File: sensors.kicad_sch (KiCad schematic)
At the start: 9 parts, among them IC4 BME690, U2 BME280, U3 BMP581

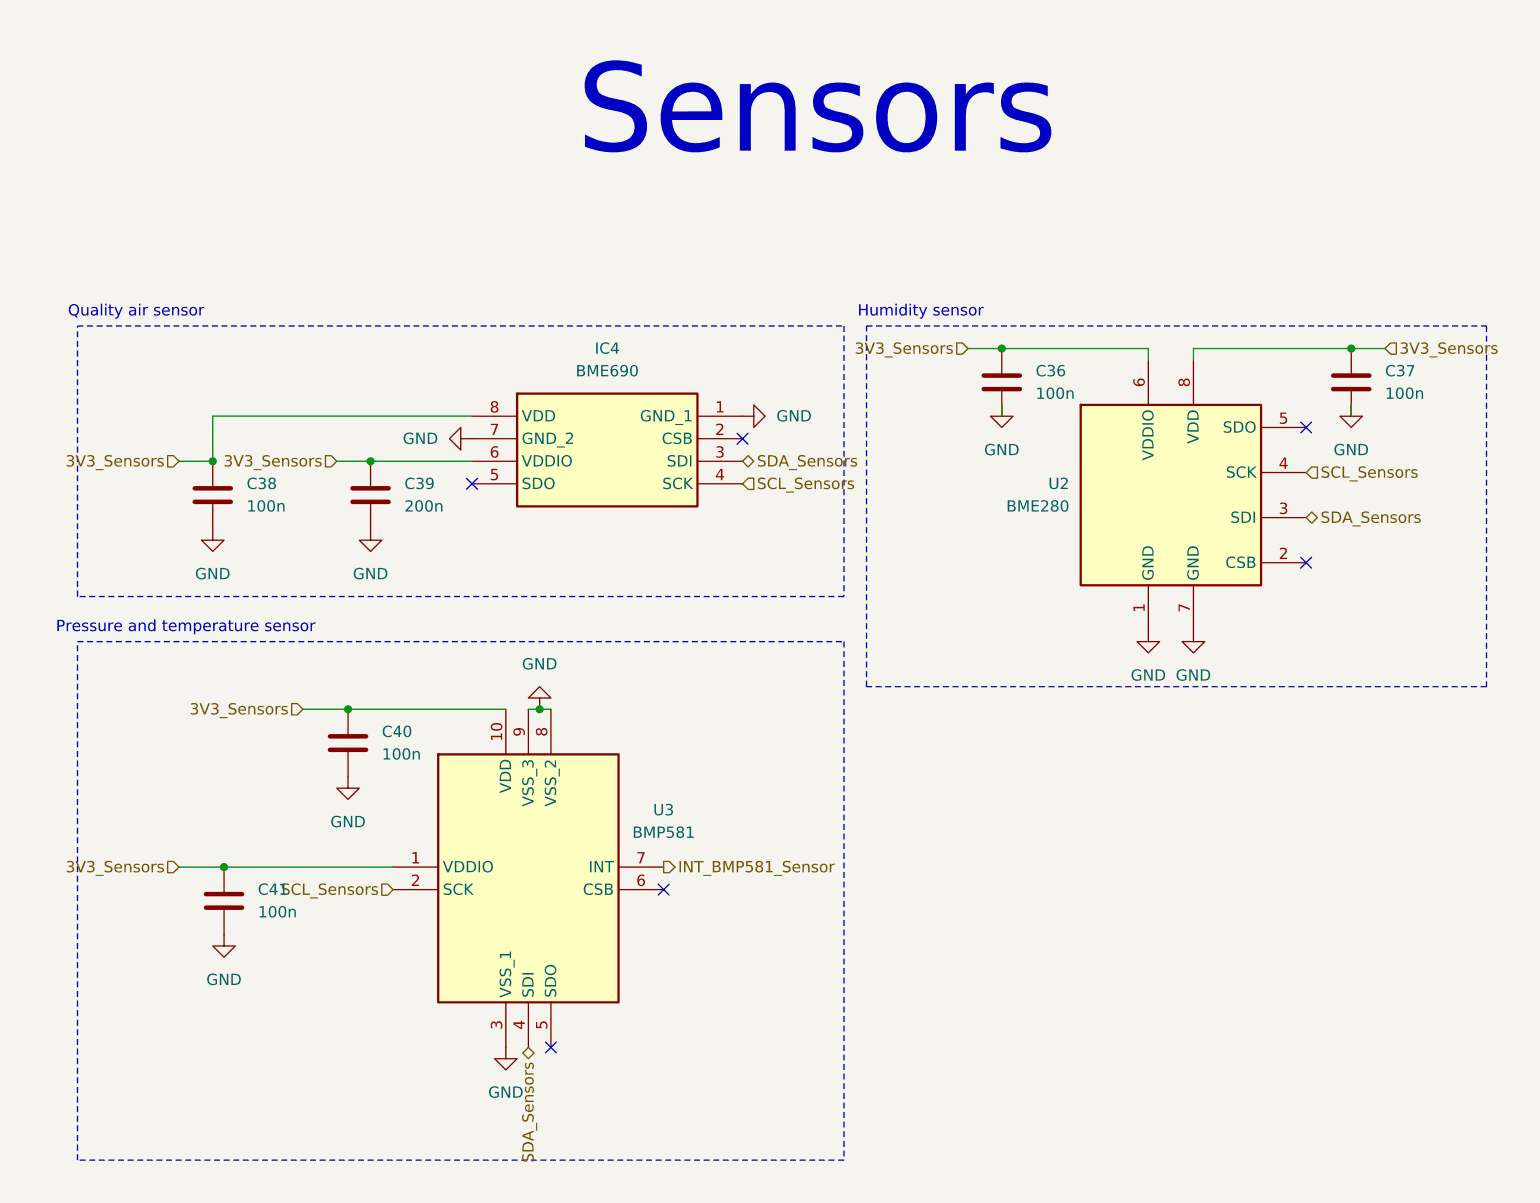
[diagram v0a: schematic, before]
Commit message: Place all components on the PCB correctly
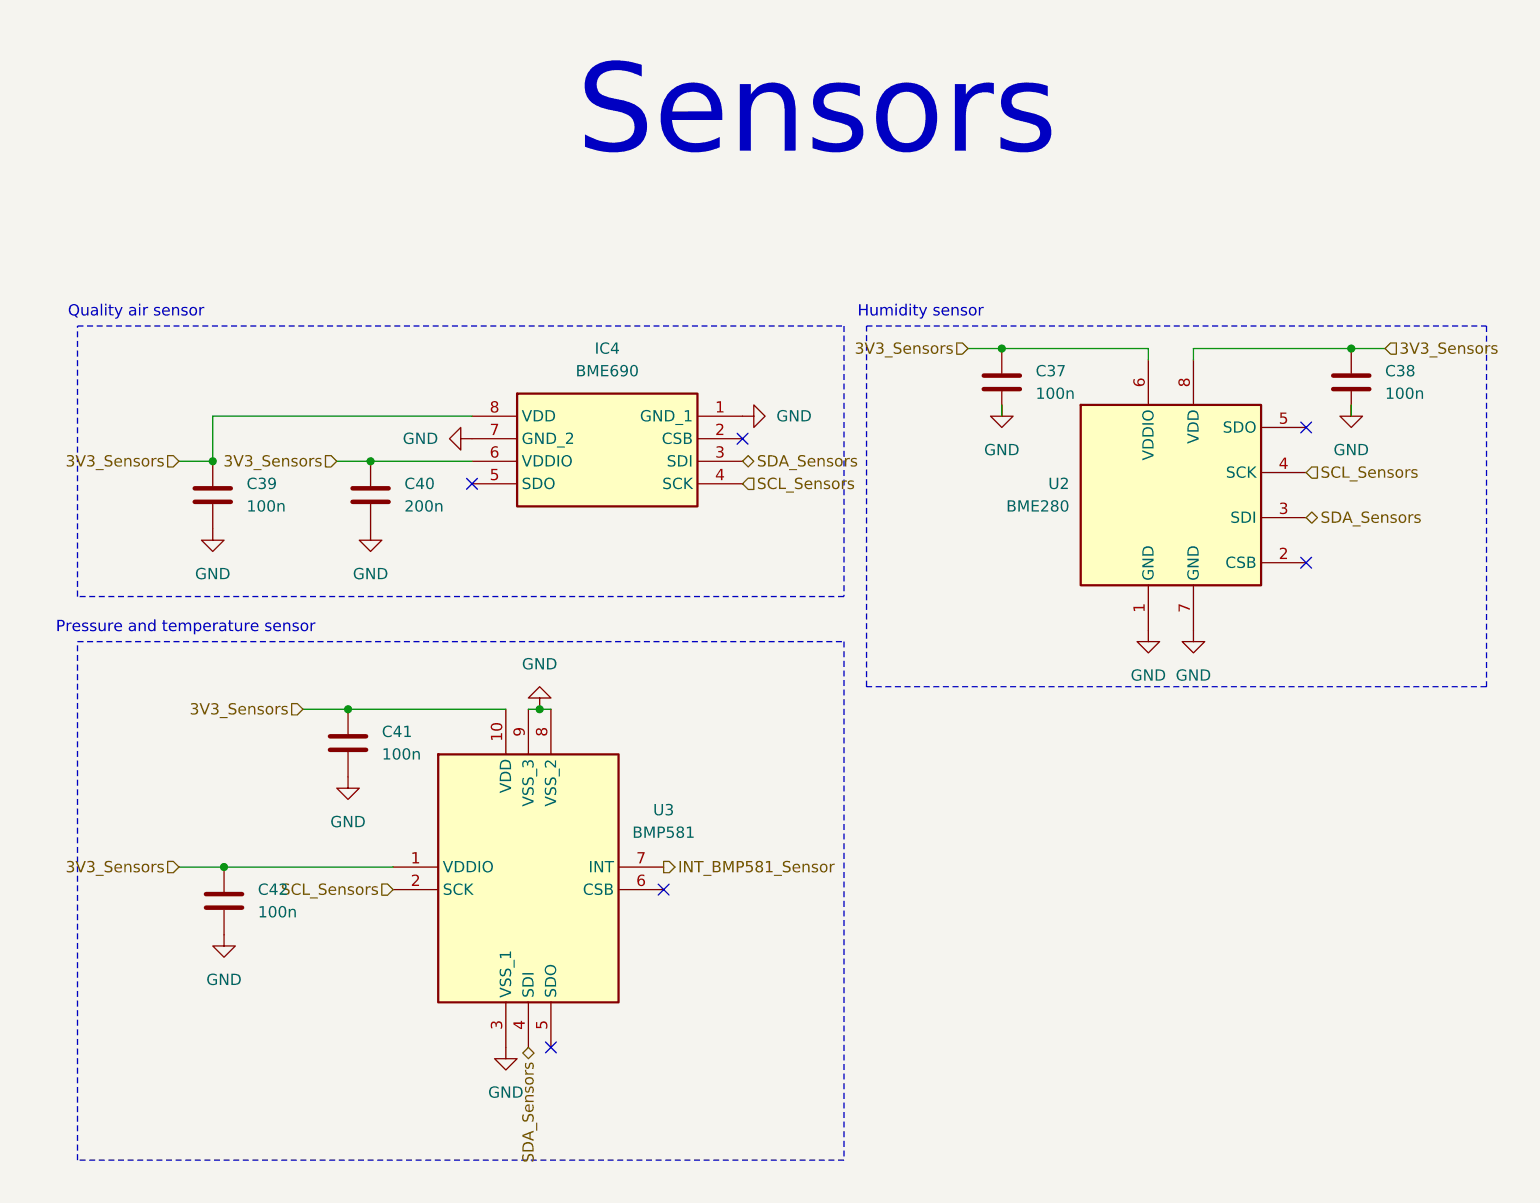
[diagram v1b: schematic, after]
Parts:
- renumbered C36 to C37, C37 to C38, C38 to C39, C39 to C40, C40 to C41, C41 to C42
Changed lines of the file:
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@@
 		(dnp no)
 		(fields_autoplaced yes)
-		(property "Reference" "#PWR058"
+		(property "Reference" "#PWR059"
 			(at 170.18 66.04 0)
 			(effects
@@
 			(project "weather-station-poc"
 				(path "/38eb53bb-294e-46e4-ad59-fd355ca373b9/29574217-d56b-4a63-a2c4-128dfec2758e"
-					(reference "#PWR058")
+					(reference "#PWR059")
 					(unit 1)
 				)
@@
 		(dnp no)
 		(fields_autoplaced yes)
-		(property "Reference" "#PWR060"
+		(property "Reference" "#PWR061"
 			(at 147.32 60.96 0)
 			(effects
@@
 			(project "weather-station-poc"
 				(path "/38eb53bb-294e-46e4-ad59-fd355ca373b9/29574217-d56b-4a63-a2c4-128dfec2758e"
-					(reference "#PWR060")
+					(reference "#PWR061")
 					(unit 1)
 				)
@@
 		(dnp no)
 		(fields_autoplaced yes)
-		(property "Reference" "C37"
+		(property "Reference" "C38"
 			(at 213.36 55.8799 0)
 			(effects
@@
 			(project "weather-station-poc"
 				(path "/38eb53bb-294e-46e4-ad59-fd355ca373b9/29574217-d56b-4a63-a2c4-128dfec2758e"
-					(reference "C37")
+					(reference "C38")
 					(unit 1)
 				)
@@
 		(dnp no)
 		(fields_autoplaced yes)
-		(property "Reference" "C38"
+		(property "Reference" "C39"
 			(at 85.09 68.5799 0)
 			(effects
@@
 			(project ""
 				(path "/38eb53bb-294e-46e4-ad59-fd355ca373b9/29574217-d56b-4a63-a2c4-128dfec2758e"
-					(reference "C38")
+					(reference "C39")
 					(unit 1)
 				)
@@
 		(dnp no)
 		(fields_autoplaced yes)
-		(property "Reference" "#PWR062"
+		(property "Reference" "#PWR063"
 			(at 81.28 80.01 0)
 			(effects
@@
 			(project ""
 				(path "/38eb53bb-294e-46e4-ad59-fd355ca373b9/29574217-d56b-4a63-a2c4-128dfec2758e"
-					(reference "#PWR062")
+					(reference "#PWR063")
 					(unit 1)
 				)
@@
 		(dnp no)
 		(fields_autoplaced yes)
-		(property "Reference" "#PWR065"
+		(property "Reference" "#PWR066"
 			(at 191.77 91.44 0)
 			(effects
@@
 			(project "weather-station-poc"
 				(path "/38eb53bb-294e-46e4-ad59-fd355ca373b9/29574217-d56b-4a63-a2c4-128dfec2758e"
-					(reference "#PWR065")
+					(reference "#PWR066")
 					(unit 1)
 				)
@@
 		(dnp no)
 		(fields_autoplaced yes)
-		(property "Reference" "#PWR066"
+		(property "Reference" "#PWR067"
 			(at 118.11 87.63 0)
 			(effects
@@
 			(project "weather-station-poc"
 				(path "/38eb53bb-294e-46e4-ad59-fd355ca373b9/29574217-d56b-4a63-a2c4-128dfec2758e"
-					(reference "#PWR066")
+					(reference "#PWR067")
 					(unit 1)
 				)
@@
 		(dnp no)
 		(fields_autoplaced yes)
-		(property "Reference" "C39"
+		(property "Reference" "C40"
 			(at 102.87 68.5799 0)
 			(effects
@@
 			(project "weather-station-poc"
 				(path "/38eb53bb-294e-46e4-ad59-fd355ca373b9/29574217-d56b-4a63-a2c4-128dfec2758e"
-					(reference "C39")
+					(reference "C40")
 					(unit 1)
 				)
@@
 		(dnp no)
 		(fields_autoplaced yes)
-		(property "Reference" "#PWR063"
+		(property "Reference" "#PWR064"
 			(at 99.06 80.01 0)
 			(effects
@@
 			(project "weather-station-poc"
 				(path "/38eb53bb-294e-46e4-ad59-fd355ca373b9/29574217-d56b-4a63-a2c4-128dfec2758e"
-					(reference "#PWR063")
+					(reference "#PWR064")
 					(unit 1)
 				)
@@
 		(dnp no)
 		(fields_autoplaced yes)
-		(property "Reference" "#PWR059"
+		(property "Reference" "#PWR060"
 			(at 209.55 66.04 0)
 			(effects
@@
 			(project "weather-station-poc"
 				(path "/38eb53bb-294e-46e4-ad59-fd355ca373b9/29574217-d56b-4a63-a2c4-128dfec2758e"
-					(reference "#PWR059")
+					(reference "#PWR060")
 					(unit 1)
 				)
@@
 		(dnp no)
 		(fields_autoplaced yes)
-		(property "Reference" "#PWR068"
+		(property "Reference" "#PWR069"
 			(at 82.55 125.73 0)
 			(effects
@@
 			(project "weather-station-poc"
 				(path "/38eb53bb-294e-46e4-ad59-fd355ca373b9/29574217-d56b-4a63-a2c4-128dfec2758e"
-					(reference "#PWR068")
+					(reference "#PWR069")
 					(unit 1)
 				)
@@
 		(dnp no)
 		(fields_autoplaced yes)
-		(property "Reference" "#PWR067"
+		(property "Reference" "#PWR068"
 			(at 96.52 107.95 0)
 			(effects
@@
 			(project "weather-station-poc"
 				(path "/38eb53bb-294e-46e4-ad59-fd355ca373b9/29574217-d56b-4a63-a2c4-128dfec2758e"
-					(reference "#PWR067")
+					(reference "#PWR068")
 					(unit 1)
 				)
@@
 		(dnp no)
 		(fields_autoplaced yes)
-		(property "Reference" "#PWR069"
+		(property "Reference" "#PWR070"
 			(at 114.3 138.43 0)
 			(effects
@@
 			(project "weather-station-poc"
 				(path "/38eb53bb-294e-46e4-ad59-fd355ca373b9/29574217-d56b-4a63-a2c4-128dfec2758e"
-					(reference "#PWR069")
+					(reference "#PWR070")
 					(unit 1)
 				)
@@
 		(dnp no)
 		(fields_autoplaced yes)
-		(property "Reference" "#PWR061"
+		(property "Reference" "#PWR062"
 			(at 104.14 63.5 0)
 			(effects
@@
 			(project "weather-station-poc"
 				(path "/38eb53bb-294e-46e4-ad59-fd355ca373b9/29574217-d56b-4a63-a2c4-128dfec2758e"
-					(reference "#PWR061")
+					(reference "#PWR062")
 					(unit 1)
 				)
@@
 		(dnp no)
 		(fields_autoplaced yes)
-		(property "Reference" "C41"
+		(property "Reference" "C42"
 			(at 86.36 114.2999 0)
 			(effects
@@
 			(project "weather-station-poc"
 				(path "/38eb53bb-294e-46e4-ad59-fd355ca373b9/29574217-d56b-4a63-a2c4-128dfec2758e"
-					(reference "C41")
+					(reference "C42")
 					(unit 1)
 				)
@@
 		(dnp no)
 		(fields_autoplaced yes)
-		(property "Reference" "#PWR064"
+		(property "Reference" "#PWR065"
 			(at 186.69 91.44 0)
 			(effects
@@
 			(project "weather-station-poc"
 				(path "/38eb53bb-294e-46e4-ad59-fd355ca373b9/29574217-d56b-4a63-a2c4-128dfec2758e"
-					(reference "#PWR064")
+					(reference "#PWR065")
 					(unit 1)
 				)
@@
 		(dnp no)
 		(fields_autoplaced yes)
-		(property "Reference" "C40"
+		(property "Reference" "C41"
 			(at 100.33 96.5199 0)
 			(effects
@@
 			(project "weather-station-poc"
 				(path "/38eb53bb-294e-46e4-ad59-fd355ca373b9/29574217-d56b-4a63-a2c4-128dfec2758e"
-					(reference "C40")
+					(reference "C41")
 					(unit 1)
 				)
@@
 		(dnp no)
 		(fields_autoplaced yes)
-		(property "Reference" "C36"
+		(property "Reference" "C37"
 			(at 173.99 55.8799 0)
 			(effects
@@
 			(project "weather-station-poc"
 				(path "/38eb53bb-294e-46e4-ad59-fd355ca373b9/29574217-d56b-4a63-a2c4-128dfec2758e"
-					(reference "C36")
-					(unit 1)
-				)
+					(reference "C37")
+					(unit 1)
+				)
